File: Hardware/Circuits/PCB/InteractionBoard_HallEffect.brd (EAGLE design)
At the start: 72.1 x 146.3 mm, 70 parts, among them J3 F-2X10-DIL-2MM, SW1 219-10, U1 DRV5032FADBZRDBZ0003A_L, U2 SX1509, U3 DRV5032FADBZRDBZ0003A_L, U4 DRV5032FADBZRDBZ0003A_L, U5 DRV5032FADBZRDBZ0003A_L, U6 DRV5032FADBZRDBZ0003A_L, U7 DRV5032FADBZRDBZ0003A_L, U8 DRV5032FADBZRDBZ0003A_L, U9 DRV5032FADBZRDBZ0003A_L

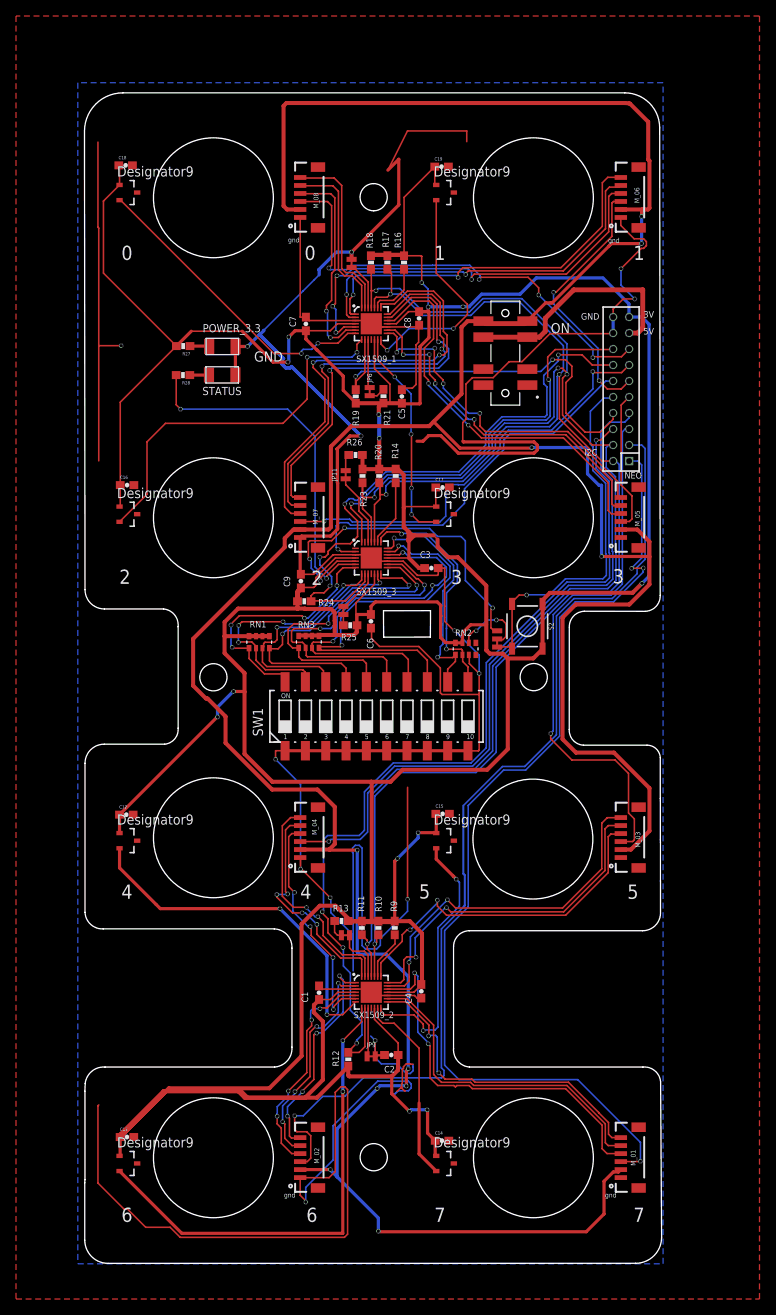
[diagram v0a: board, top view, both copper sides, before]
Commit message: manually routed
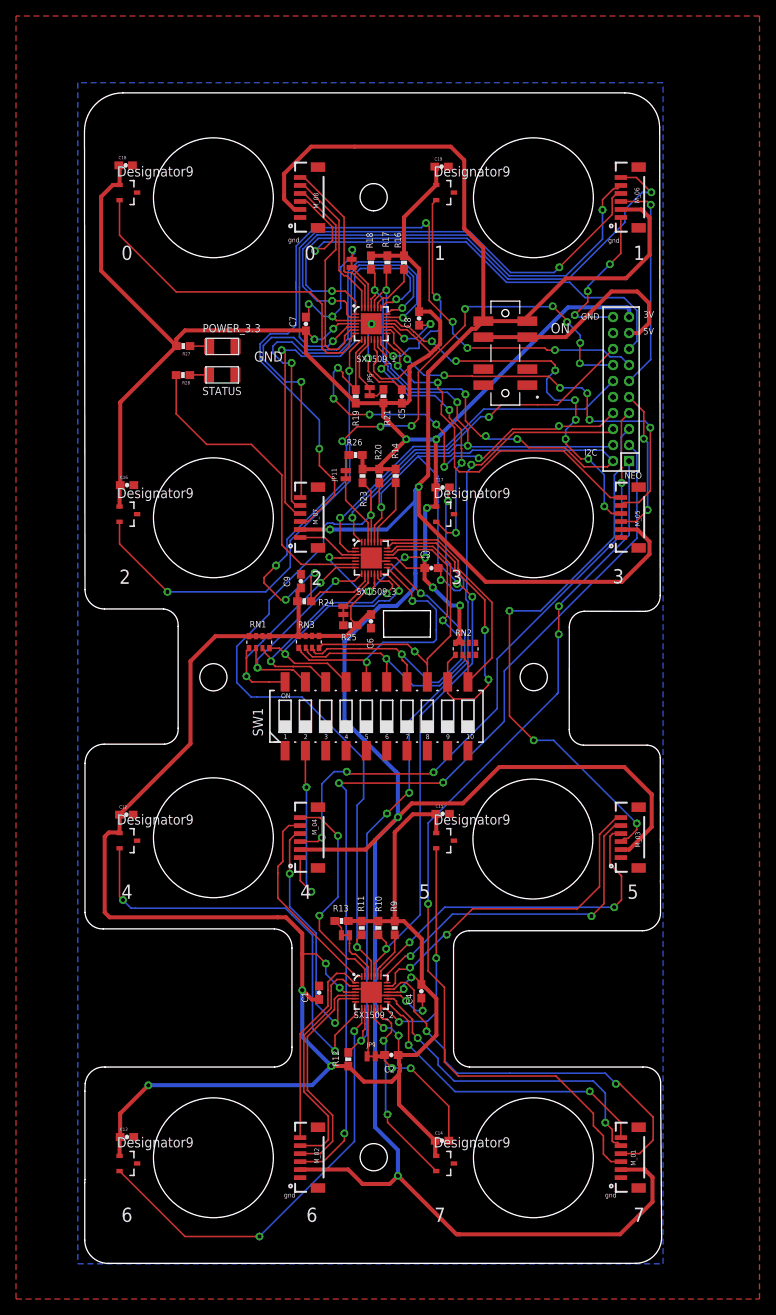
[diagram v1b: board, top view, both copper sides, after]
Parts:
- removed JP1: JUMPER-SMT_3_1-NC_TRACE_NO-SILK, SparkFun-Jumpers:SMT-JUMPER_3_1-NC_TRACE_NO-SILK
- removed S2: (no value), SparkFun-Switches:TACTILE_SWITCH_SMD_5.2MM
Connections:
- net 3.3V: no longer S2.1, S2.2
- net 4_SX3: no longer JP1.1
- net GND_MCU: no longer RN2.3
- net RESET: no longer JP1.2, JP1.3, RN2.6, S2.3, S2.4
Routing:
- net GND_MCU: track 601.2 -> 144.2 mm, vias 14 -> 18
- net 3.3V: track 749.4 -> 511.3 mm, vias 14 -> 20
- net RESET: track 56.3 -> 0.00 mm, vias 3 -> 0
- net NEOPIXEL_07: track 53.7 -> 101.3 mm, vias 2 -> 5
- net 4_SX3: track 45.8 -> 0.00 mm, vias 4 -> 0
- net VCC_5V: track 415.8 -> 382.2 mm, vias 10 -> 4
- net SCL_00: track 188.4 -> 156.0 mm
- net 2_SX2: track 47.7 -> 68.8 mm
- net INT_03: track 74.2 -> 94.0 mm, vias 4 -> 11
- net 3_SX2: track 47.9 -> 63.9 mm
- net 4_SX2: track 54.4 -> 68.1 mm, vias 4 -> 2
- net SDA_00: track 181.0 -> 167.7 mm, vias 4 -> 8
- net 7_SX2: track 47.2 -> 60.1 mm
- net INT_01: track 115.6 -> 104.1 mm
- net NEOPIXEL_01: track 126.8 -> 115.9 mm
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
